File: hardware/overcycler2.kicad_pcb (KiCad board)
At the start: 2 copper layers, 208.3 x 152.4 mm, 276 parts, among them IC1 LM13700, IC2 LM13700, IC3 LM13700, P1 LPC_P1, P2 LPC_P2, P3 FT232, P4 PANEL, P5 SDCARD, P6 MIDI_IN, P7 FOOT_IN, P8 AC_IN, P9 AUDIO_OUT, Q1 BC547, SW1 RESET, U1 TLV1543, U10 MCP4922-E/P, U11 SSM2044, U12 MCP4922-E/P, U13 SSM2044, U14 MCP4922-E/P, U15 SSM2044, U16 MCP4922-E/P, U17 SSM2044, U18 MCP4922-E/P, U19 SSM2044, U2 74HC138, U20 MCP4922-E/P, U21 SSM2044, U3 LTC1660, U4 LTC1660, U5 TL074, U6 TL074, U7 LM1084IT-5.0/NOPB, U8 LM2990-5.0/NOPB, U9 LM1084IT-ADJ/NOPB

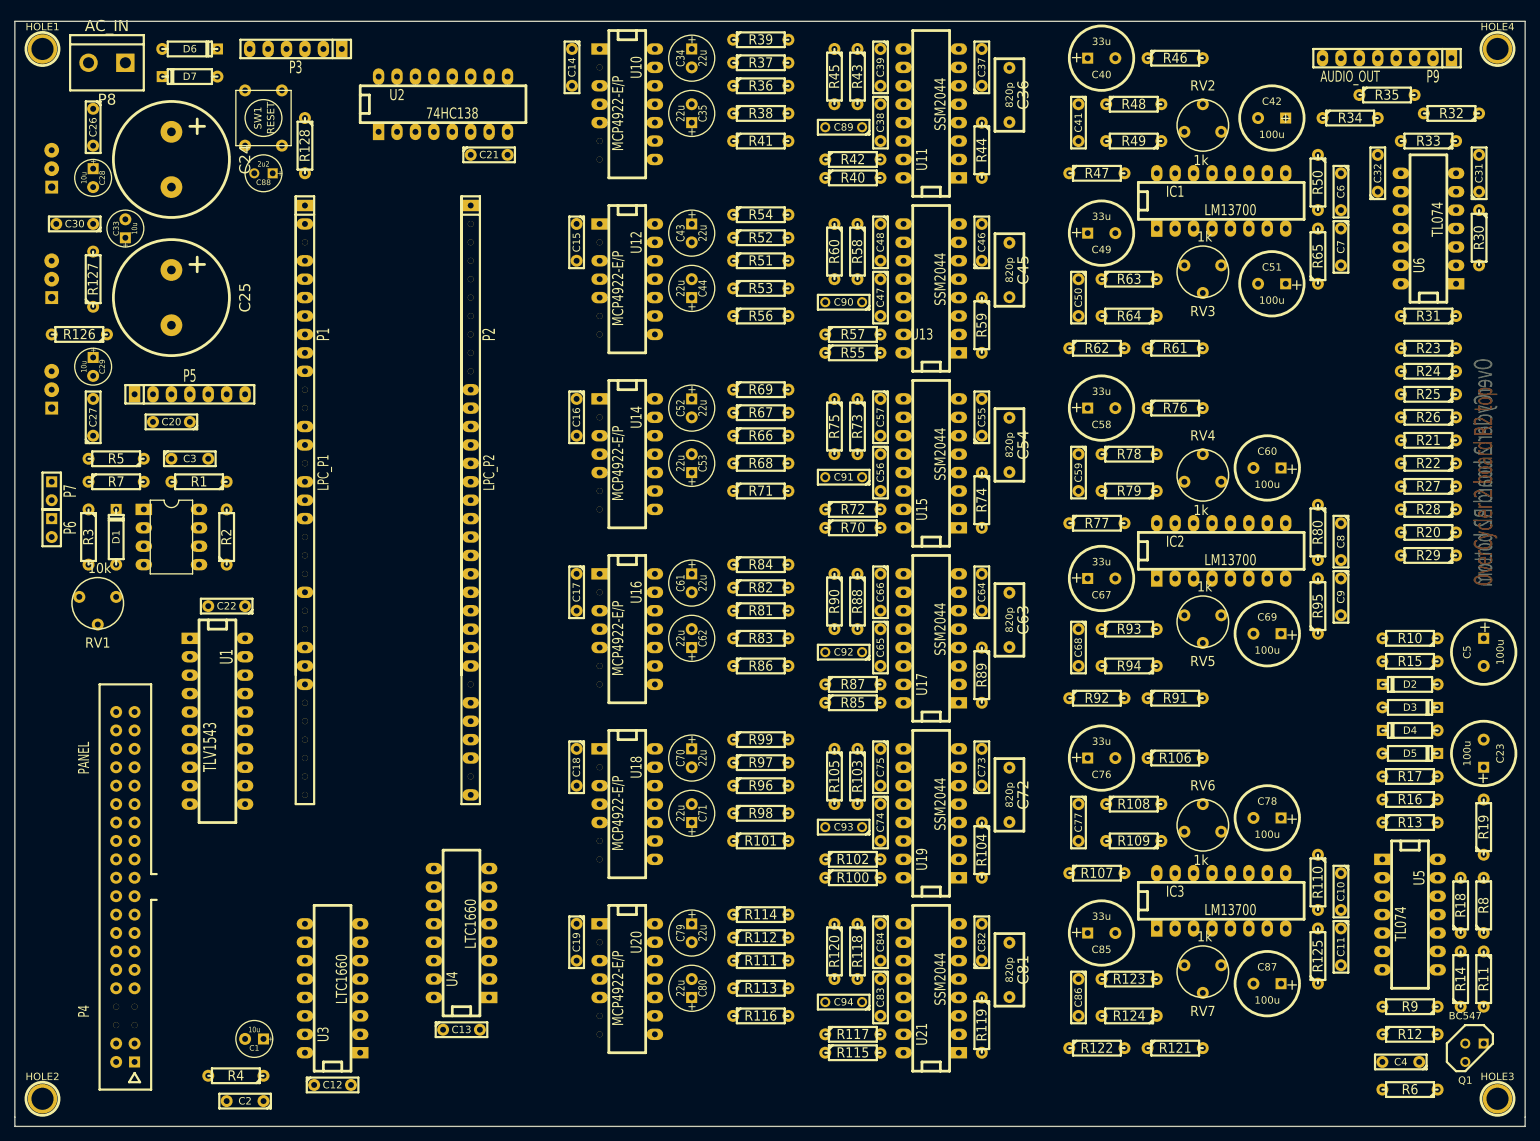
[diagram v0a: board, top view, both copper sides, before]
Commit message: rev3 pcb
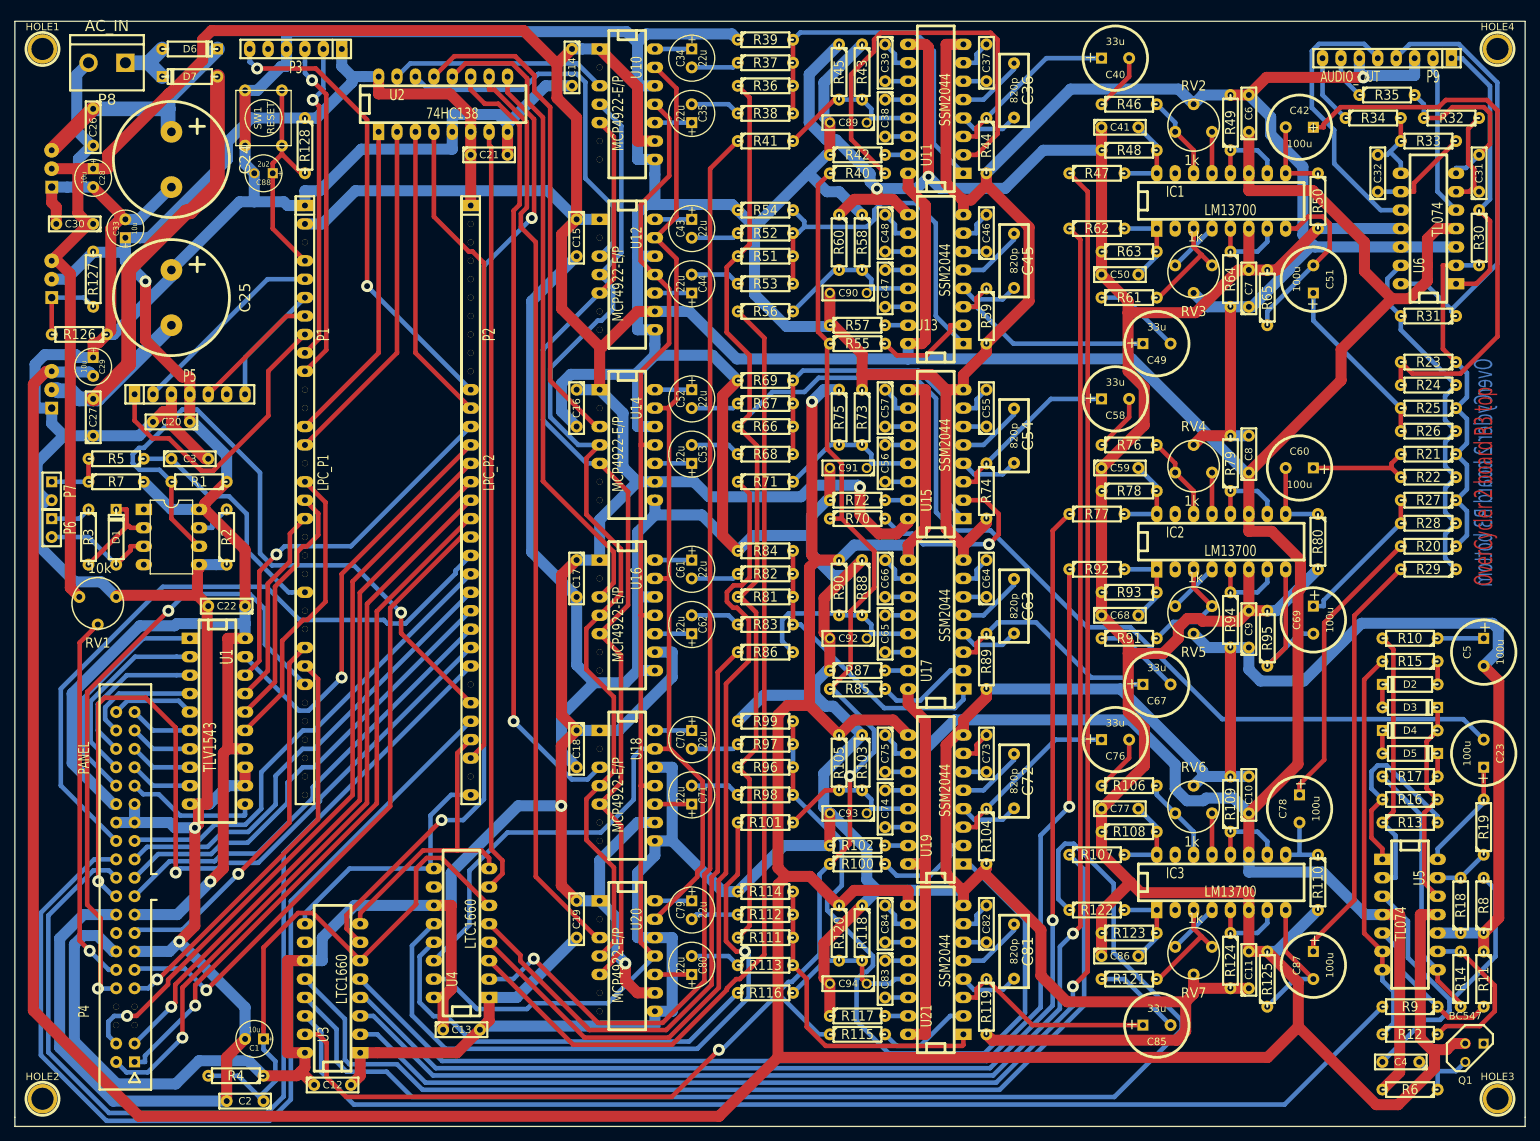
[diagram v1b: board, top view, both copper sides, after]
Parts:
- moved R122 19.0 mm to (174.6, 148.0)
- moved C10 18.4 mm to (195.6, 132.1), turned to 90 degrees
- moved R92 17.8 mm to (174.6, 101.0)
- moved C8 17.5 mm to (195.6, 85.1), turned to 90 degrees
- moved C49 17.0 mm to (182.9, 69.8)
- moved C6 16.7 mm to (195.6, 38.1), turned to 90 degrees
- moved R62 16.5 mm to (174.6, 54.0)
- moved C67 16.5 mm to (182.9, 116.8)
- moved R124 15.9 mm to (193.0, 154.9), turned to 270 degrees
- moved R94 15.3 mm to (193.0, 108.0), turned to 270 degrees
- moved R64 14.9 mm to (193.0, 61.0), turned to 270 degrees
- moved C85 14.8 mm to (182.9, 163.8)
- moved R79 14.5 mm to (193.0, 86.4), turned to 90 degrees
- moved R109 14.3 mm to (193.0, 133.3), turned to 90 degrees
- moved C7 13.9 mm to (195.6, 62.2), turned to 90 degrees
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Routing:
- net GND: track 0.00 -> 1701.5 mm, vias 0 -> 3
- net +5V: track 0.00 -> 1051.7 mm, vias 0 -> 3
- net -5V: track 0.00 -> 873.3 mm, vias 0 -> 3
- net +3.3V: track 0.00 -> 264.0 mm, vias 0 -> 2
- net NOISE: track 0.00 -> 262.7 mm
- net /Voice #0/DAC_VCA: track 0.00 -> 222.2 mm, vias 0 -> 1
- net DAC_RES: track 0.00 -> 217.0 mm, vias 0 -> 2
- net /Voice #1/DAC_VCA: track 0.00 -> 213.1 mm, vias 0 -> 1
- net DAC_MIXA: track 0.00 -> 182.6 mm
- net /Voice #5/DAC_VCA: track 0.00 -> 176.2 mm
- net /Voice #2/DAC_VCA: track 0.00 -> 171.8 mm, vias 0 -> 1
- net DAC_MIXB: track 0.00 -> 165.1 mm
- net /Voice #3/DAC_VCA: track 0.00 -> 163.6 mm, vias 0 -> 1
- net /DAC_MIXN: track 0.00 -> 162.5 mm
- net /Voice #0/DAC_FC: track 0.00 -> 154.7 mm, vias 0 -> 1
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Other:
- board text added: "OverCycler 2 board R3 bottom"
- board text added: "OverCycler 2 board R3 top"
- board text removed: "OverCycler 2 board R2 bottom"
- board text removed: "OverCycler 2 board R2 top"
